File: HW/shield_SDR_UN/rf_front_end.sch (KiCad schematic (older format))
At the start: 80 parts, among them Q1 MOSFET_P, U1 MAX5864, U2 MAX2830

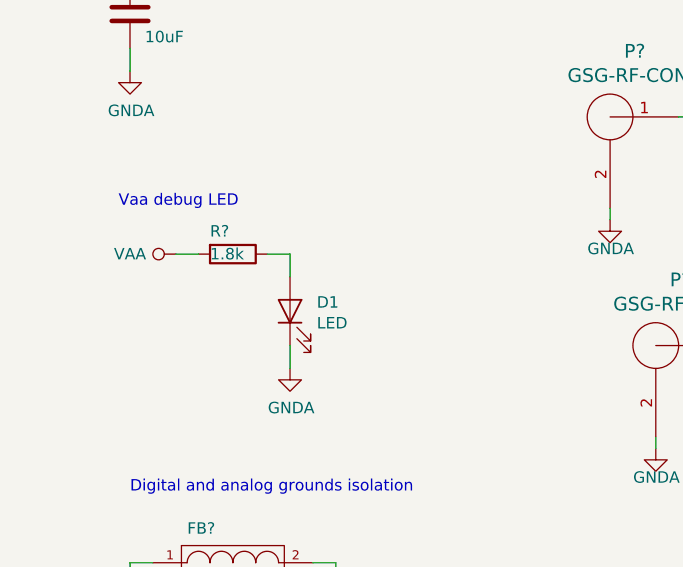
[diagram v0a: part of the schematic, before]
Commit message: Footprints updated
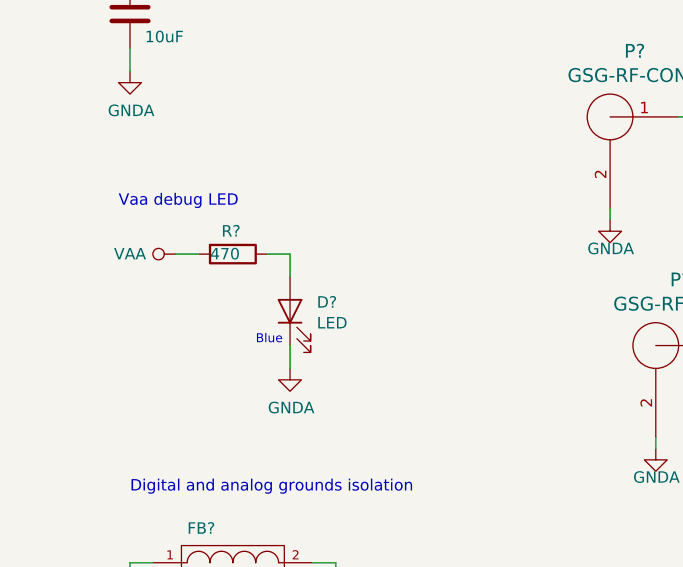
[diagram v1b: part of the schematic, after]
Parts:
- removed D1: LED, symbol Device:LED
- removed R?: 1.8k, Resistor_SMD:R_0603_1608Metric_Pad1.05x0.95mm_HandSolder, symbol Device:R
- added D?: LED, LED_SMD:LED_0805_2012Metric_Pad1.15x1.40mm_HandSolder, symbol Device:LED
- added R?: 470, Resistor_SMD:R_0603_1608Metric_Pad1.05x0.95mm_HandSolder, symbol Device:R
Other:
- note added: "Blue"
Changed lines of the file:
@@
-	0    -1   -1   0
-$EndComp
-$Comp
-L Device:LED D1
-U 1 1 5CE581D2
-P 1950 4250
-F 0 "D1" V 1989 4133 50  0000 R CNN
-F 1 "LED" V 1898 4133 50  0000 R CNN
-F 2 "" H 1950 4250 50  0001 C CNN
-F 3 "~" H 1950 4250 50  0001 C CNN
-	1    1950 4250
 	0    -1   -1   0
 $EndComp
@@
 $Comp
 L Device:R R?
-U 1 1 5CFC6C9A
+U 1 1 5CEDD000
 P 1700 4000
-F 0 "R?" V 1600 3900 50  0000 L CNN
-F 1 "1.8k" V 1700 3900 50  0000 L CNN
+F 0 "R?" V 1600 3950 50  0000 L CNN
+F 1 "470" V 1700 3900 50  0000 L CNN
 F 2 "Resistor_SMD:R_0603_1608Metric_Pad1.05x0.95mm_HandSolder" V 1630 4000 50  0001 C CNN
 F 3 "http://www.yageo.com/documents/recent/PYu-RC_Group_51_RoHS_L_10.pdf" H 1700 4000 50  0001 C CNN
-F 4 "311-1.8KGRTR-ND" V 1700 4000 50  0001 C CNN "Digikey"
+F 4 "311-470GRCT-ND" V 1700 4000 50  0001 C CNN "Digikey"
 	1    1700 4000
 	0    1    1    0
 $EndComp
+Text Notes 1800 4400 0    39   ~ 0
+Blue
+$Comp
+L Device:LED D?
+U 1 1 5CEDF6C9
+P 1950 4250
+AR Path="/5CC082AD/5CEDF6C9" Ref="D?"  Part="1"
+AR Path="/5CFB52DC/5CEDF6C9" Ref="D?"  Part="1"
+AR Path="/5CC081D2/5CEDF6C9" Ref="D?"  Part="1"
+F 0 "D?" V 1989 4133 50  0000 R CNN
+F 1 "LED" V 1898 4133 50  0000 R CNN
+F 2 "LED_SMD:LED_0805_2012Metric_Pad1.15x1.40mm_HandSolder" H 1950 4250 50  0001 C CNN
+F 3 "http://optoelectronics.liteon.com/upload/download/DS22-2000-239/LTST-S220TBKT.pdf" H 1950 4250 50  0001 C CNN
+F 4 "160-2032-1-ND" V 1950 4250 50  0001 C CNN "Digikey"
+	1    1950 4250
+	0    -1   -1   0
+$EndComp
 Wire Bus Line
